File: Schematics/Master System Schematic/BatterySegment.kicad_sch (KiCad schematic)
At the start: 148 parts

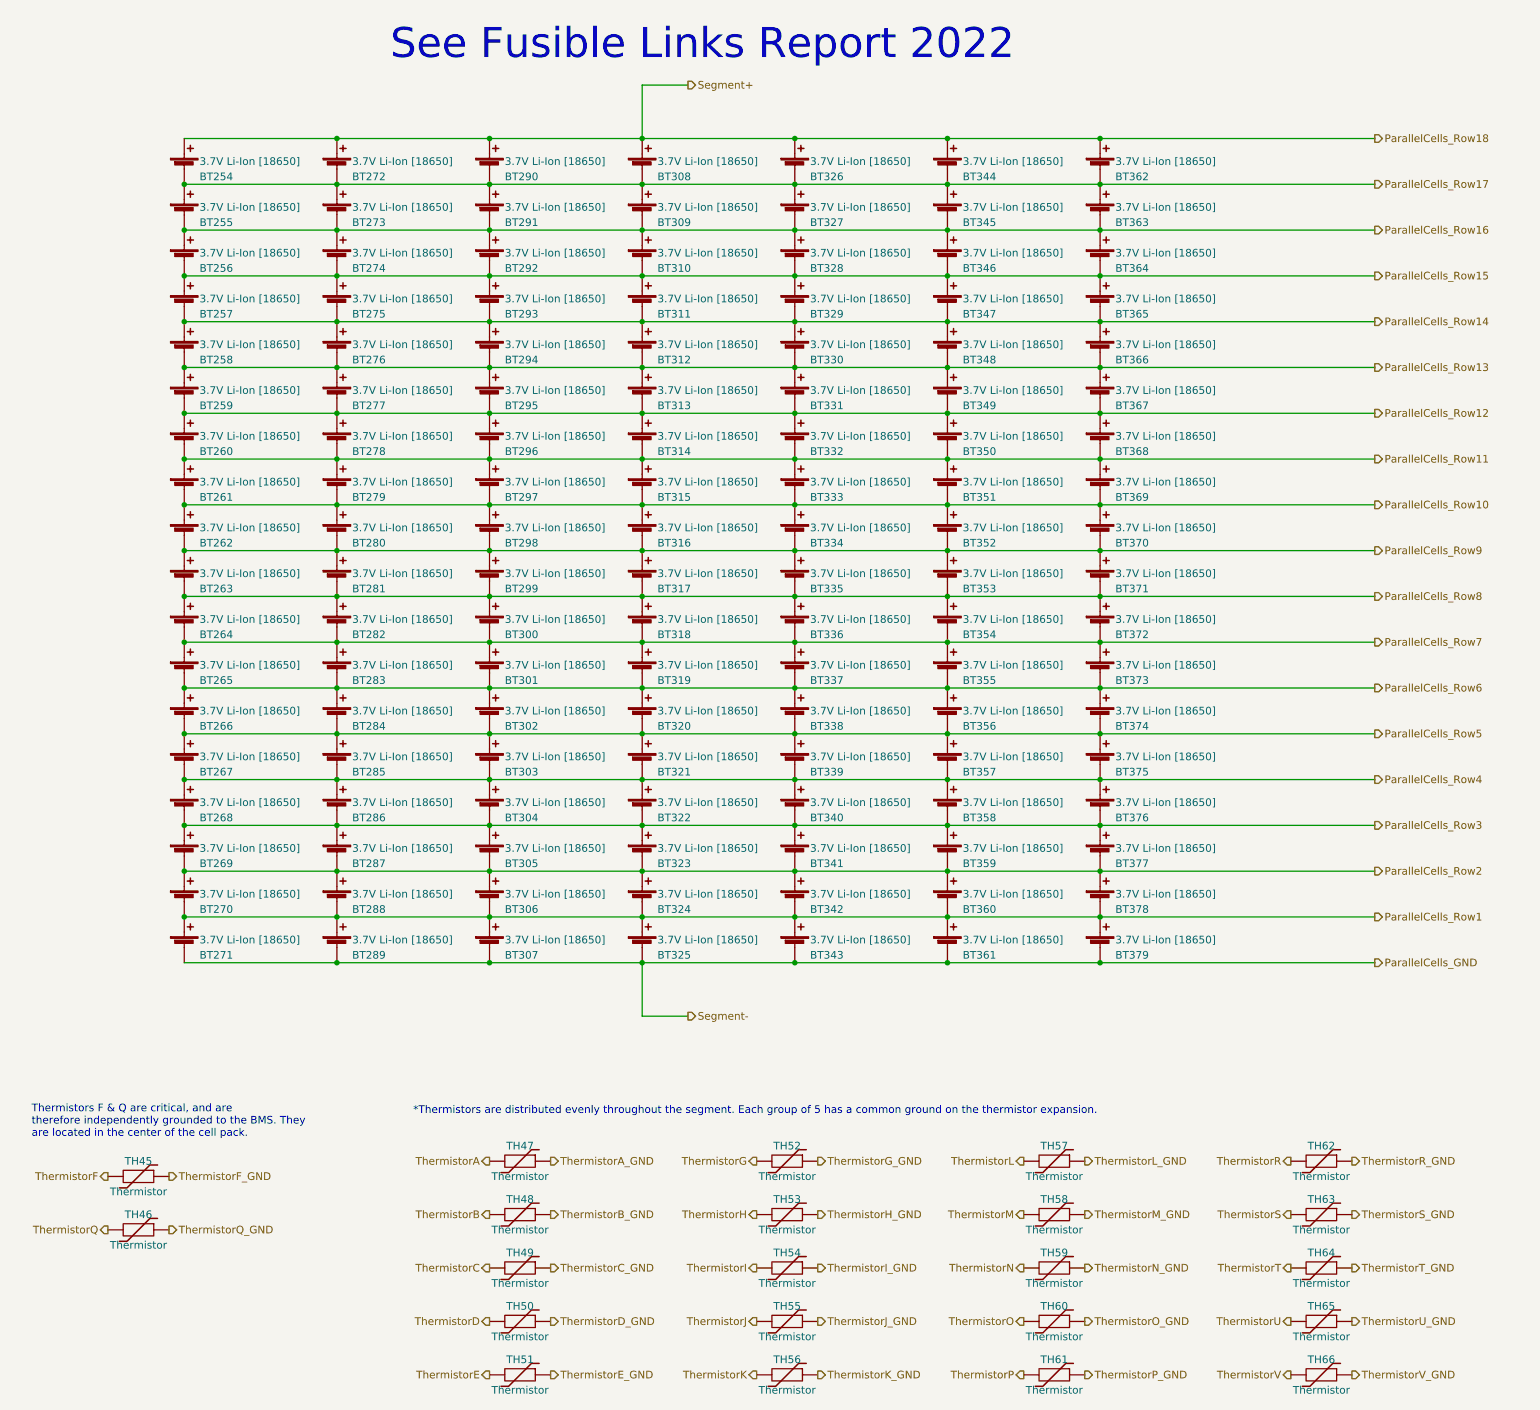
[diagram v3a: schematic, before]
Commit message: more update
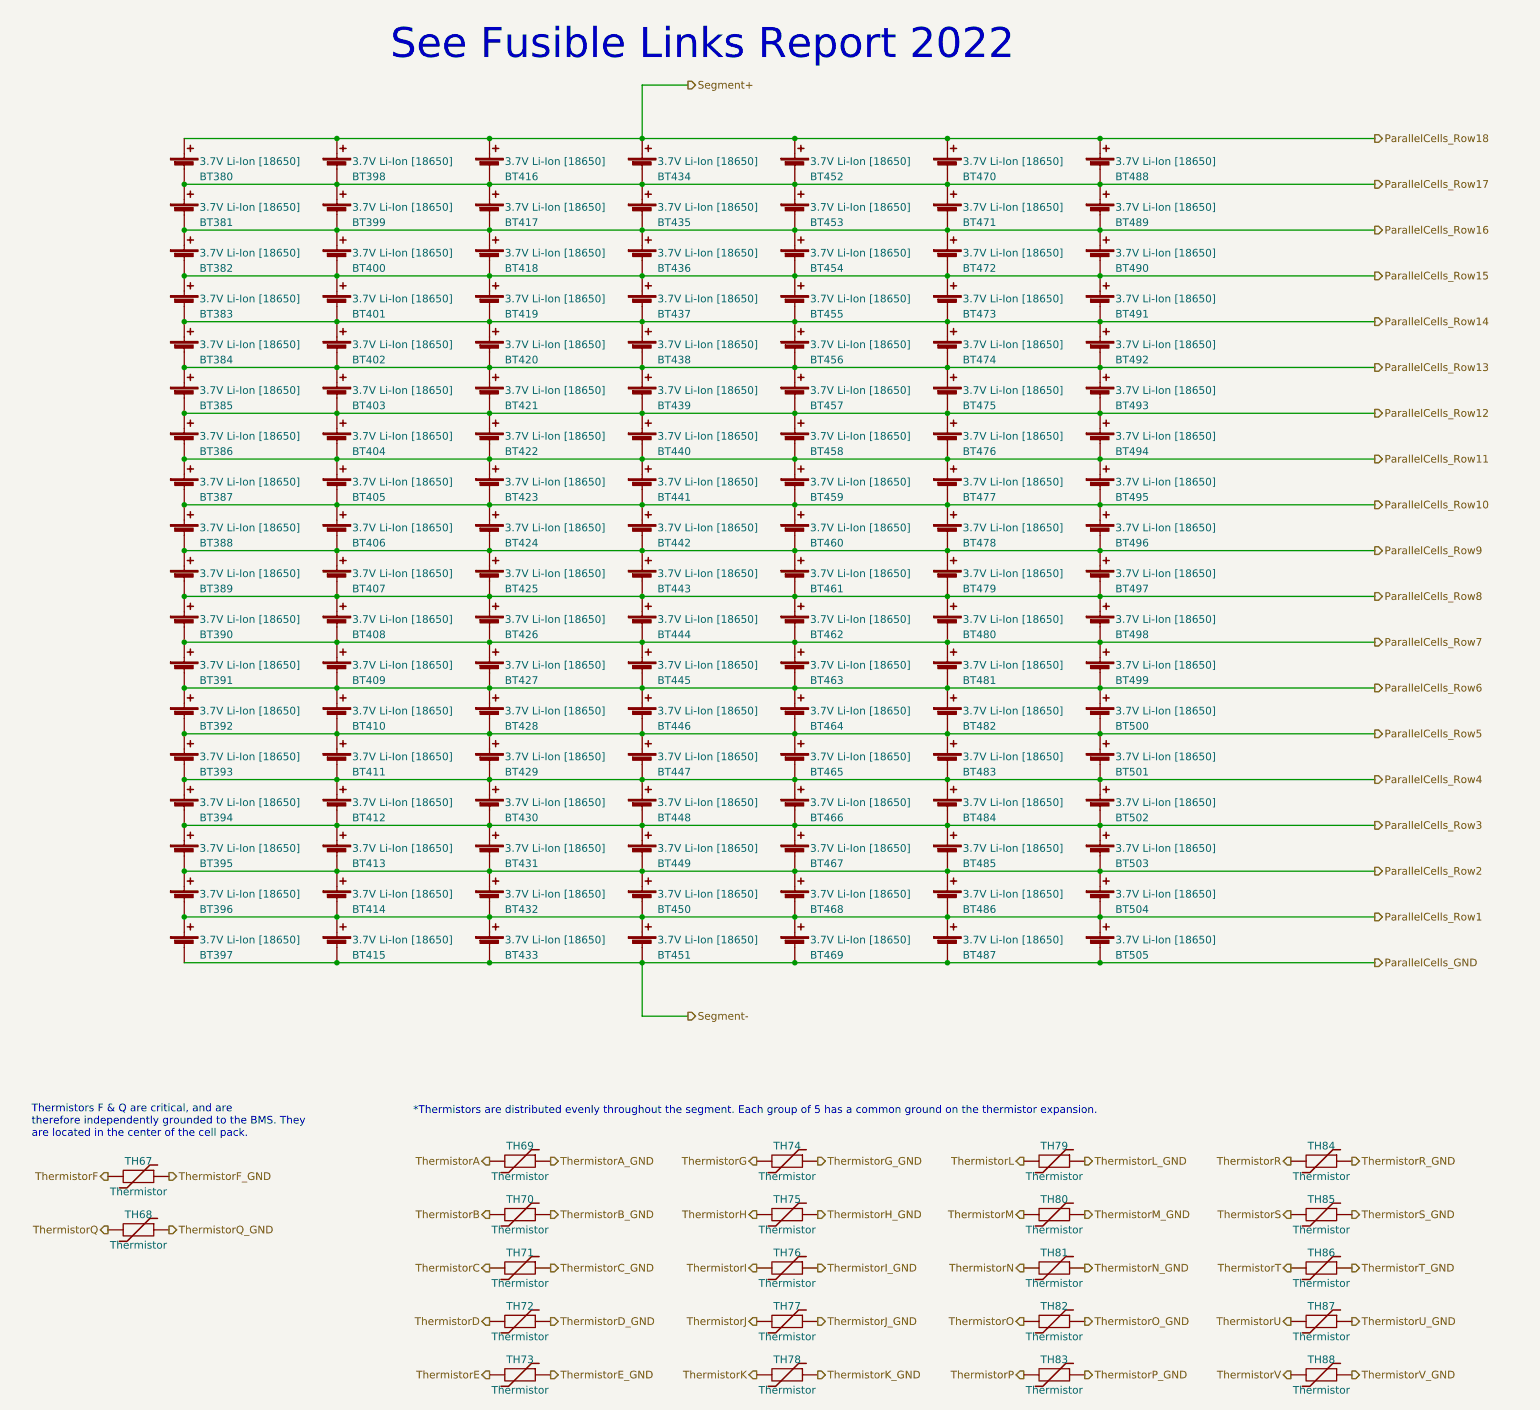
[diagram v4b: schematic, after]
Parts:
- renumbered BT254 to BT380, BT255 to BT381, BT256 to BT382, BT257 to BT383, BT258 to BT384, BT259 to BT385, BT260 to BT386, BT261 to BT387, BT262 to BT388, BT263 to BT389, BT264 to BT390, BT265 to BT391, BT266 to BT392, BT267 to BT393, BT268 to BT394, BT269 to BT395, BT270 to BT396, BT271 to BT397, BT272 to BT398, BT273 to BT399, BT274 to BT400, BT275 to BT401, BT276 to BT402, BT277 to BT403, BT278 to BT404, BT279 to BT405, BT280 to BT406, BT281 to BT407, BT282 to BT408, BT283 to BT409, BT284 to BT410, BT285 to BT411, BT286 to BT412, BT287 to BT413, BT288 to BT414, BT289 to BT415, BT290 to BT416, BT291 to BT417, BT292 to BT418, BT293 to BT419, BT294 to BT420, BT295 to BT421, BT296 to BT422, BT297 to BT423, BT298 to BT424, BT299 to BT425, BT300 to BT426, BT301 to BT427, BT302 to BT428, BT303 to BT429, BT304 to BT430, BT305 to BT431, BT306 to BT432, BT307 to BT433, BT308 to BT434, BT309 to BT435, BT310 to BT436, BT311 to BT437, BT312 to BT438, BT313 to BT439, BT314 to BT440, BT315 to BT441, BT316 to BT442, BT317 to BT443, BT318 to BT444, BT319 to BT445, BT320 to BT446, BT321 to BT447, BT322 to BT448, BT323 to BT449, BT324 to BT450, BT325 to BT451, BT326 to BT452, BT327 to BT453, BT328 to BT454, BT329 to BT455, BT330 to BT456, BT331 to BT457, BT332 to BT458, BT333 to BT459, BT334 to BT460, BT335 to BT461, BT336 to BT462, BT337 to BT463, BT338 to BT464, BT339 to BT465, BT340 to BT466, BT341 to BT467, BT342 to BT468, BT343 to BT469, BT344 to BT470, BT345 to BT471, BT346 to BT472, BT347 to BT473, BT348 to BT474, BT349 to BT475, BT350 to BT476, BT351 to BT477, BT352 to BT478, BT353 to BT479, BT354 to BT480, BT355 to BT481, BT356 to BT482, BT357 to BT483, BT358 to BT484, BT359 to BT485, BT360 to BT486, BT361 to BT487, BT362 to BT488, BT363 to BT489, BT364 to BT490, BT365 to BT491, BT366 to BT492, BT367 to BT493, BT368 to BT494, BT369 to BT495, BT370 to BT496, BT371 to BT497, BT372 to BT498, BT373 to BT499, BT374 to BT500, BT375 to BT501, BT376 to BT502, BT377 to BT503, BT378 to BT504, BT379 to BT505, TH45 to TH67, TH46 to TH68, TH47 to TH69, TH48 to TH70, TH49 to TH71, TH50 to TH72, TH51 to TH73, TH52 to TH74, TH53 to TH75, TH54 to TH76, TH55 to TH77, TH56 to TH78, TH57 to TH79, TH58 to TH80, TH59 to TH81, TH60 to TH82, TH61 to TH83, TH62 to TH84, TH63 to TH85, TH64 to TH86, TH65 to TH87, TH66 to TH88
